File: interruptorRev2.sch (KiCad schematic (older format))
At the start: 18 parts, among them J1 220v, J2 Conn_01x04, J3 Screw_Terminal_01x03, J4 Screw_Terminal_01x03, J7 Conn_01x02, Q1 2N7002, Q2 2N7002, U1 HLK-PM01, U3 ESP-07v2, U4 JRC-21(4100), U5 JRC-21(4100)

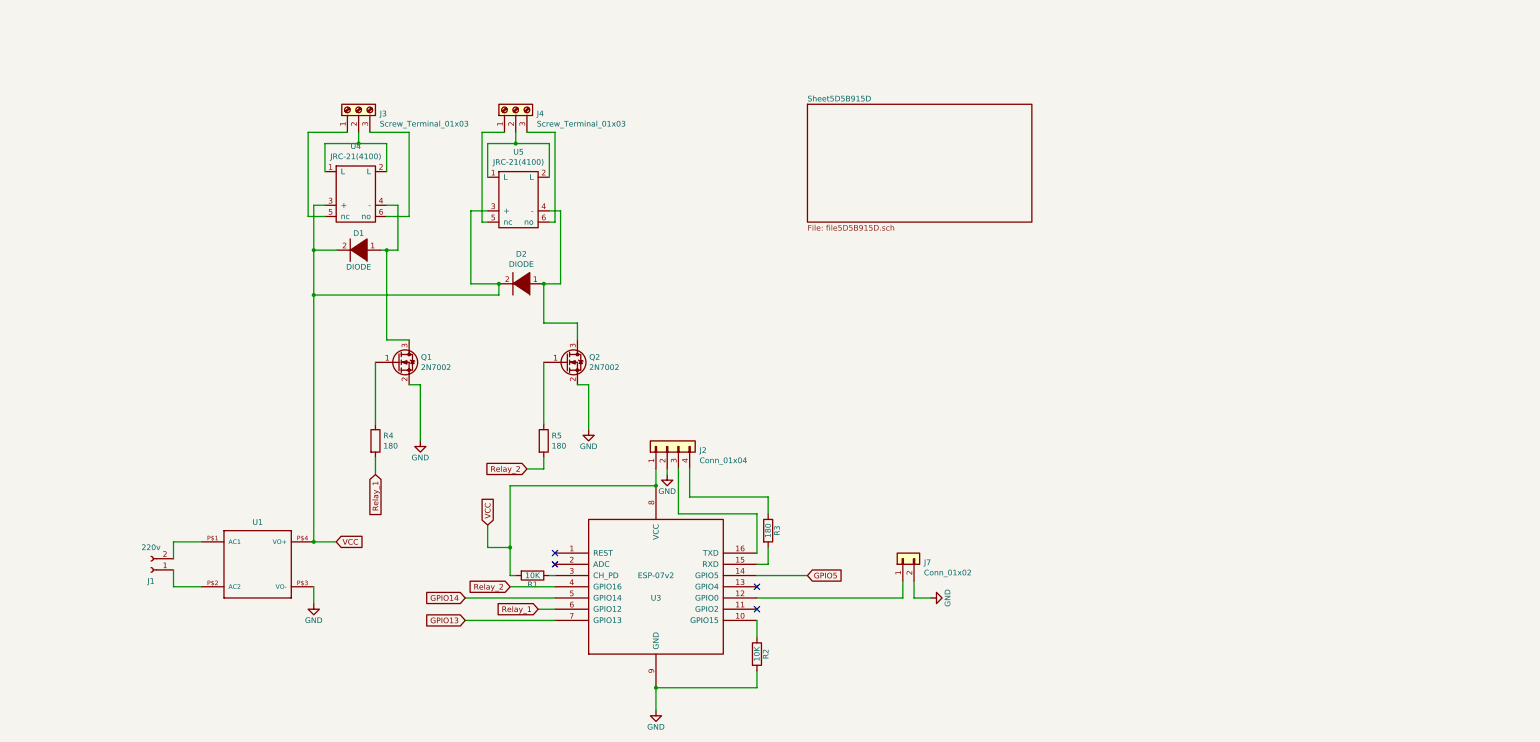
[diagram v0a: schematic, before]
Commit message: esquema dividido por secciones
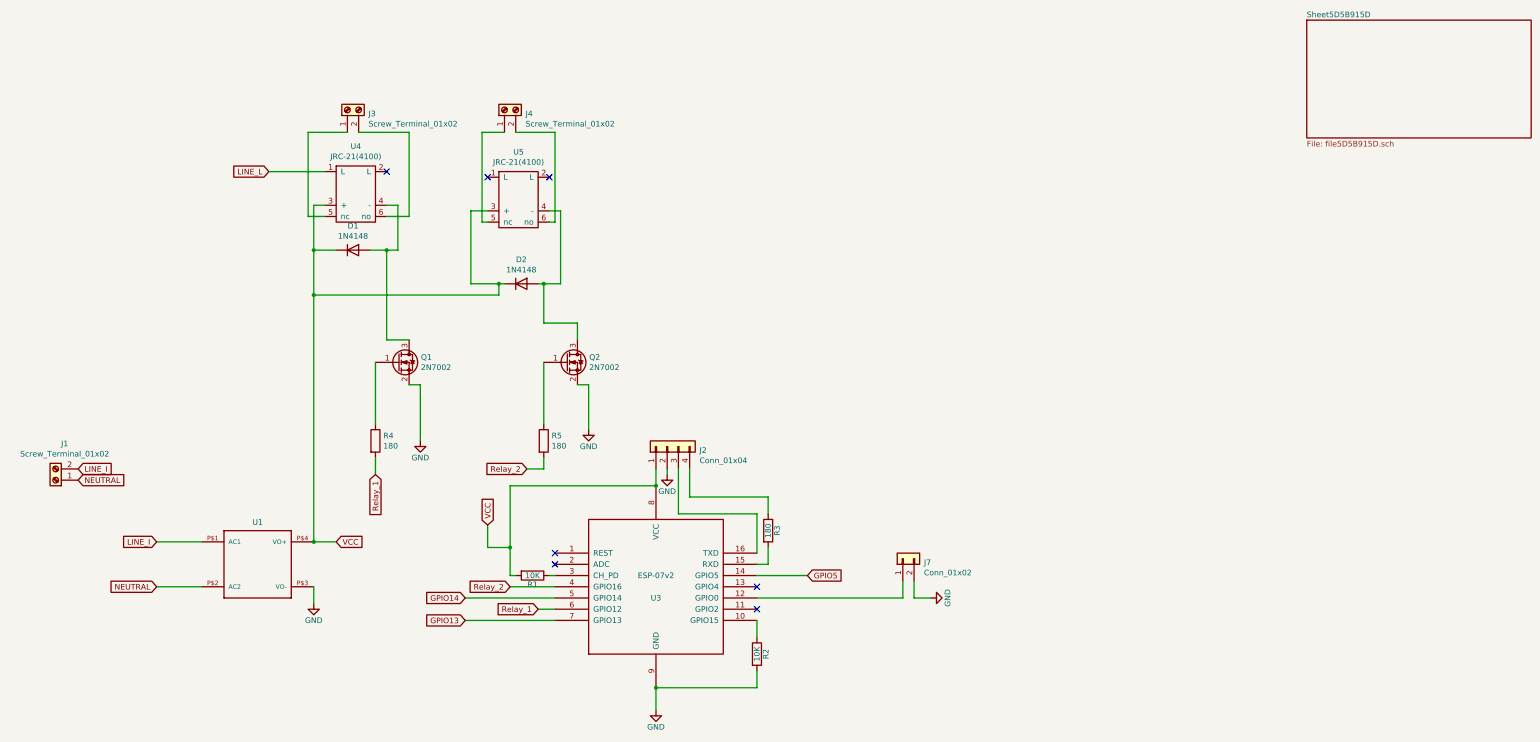
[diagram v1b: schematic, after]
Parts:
- removed D1, D2: DIODE, Diode_SMD:D_1206_3216Metric_Pad1.42x1.75mm_HandSolder, symbol pspice:DIODE
- removed J1: 220v, TerminalBlock:TerminalBlock_bornier-2_P5.08mm, symbol interruptorRev2-rescue:Conn_01x02_Female-RESCUE-termostato-termostato-rescue-in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
- removed J3, J4: Screw_Terminal_01x03, TerminalBlock:TerminalBlock_bornier-3_P5.08mm, symbol Connector:Screw_Terminal_01x03
- added D1, D2: 1N4148, espurna-h:SOD80, symbol Diode:1N4148
- added J1, J3, J4: Screw_Terminal_01x02, symbol Connector:Screw_Terminal_01x02
- R1, R2, R3, R4, R5: footprint Resistor_SMD:R_1206_3216Metric_Pad1.42x1.75mm_HandSolder -> Resistor_SMD:R_0805_2012Metric_Pad1.15x1.40mm_HandSolder
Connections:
- net VCC: now also D1.1 (K), D2.1 (K)
- net NEUTRAL: now reaches U1.P$2 (AC2)
- net NEUTRAL: now also J1.1 (Pin_1)
- net LINE_I: now reaches U1.P$1 (AC1)
- net LINE_I: now also J1.2 (Pin_2)
- net at Q1.3 (D), U4.4 (-): now also D1.2 (A)
- net at Q2.3 (D), U5.4 (-): now also D2.2 (A)
- net at U4.5 (nc): now also J3.1 (Pin_1)
- net at U4.2 (L): no longer U4.1 (L)
- net at U4.6 (no): now also J3.2 (Pin_2)
- net at U5.5 (nc): now also J4.1 (Pin_1)
- net at U5.1 (L): no longer U5.2 (L)
- net at U5.6 (no): now also J4.2 (Pin_2)
- new net LINE_L: U4.1 (L)
- no-connect marks 4 -> 7
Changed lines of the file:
@@
 Comment4 ""
 $EndDescr
-$Comp
-L interruptorRev2-rescue:Conn_01x02_Female-RESCUE-termostato-termostato-rescue-interruptor-rescue J1
-U 1 1 5A3E8B13
-P 2300 5000
-F 0 "J1" H 2300 5100 50  0000 C CNN
-F 1 "220v" H 2300 4800 50  0000 C CNN
-F 2 "TerminalBlock:TerminalBlock_bornier-2_P5.08mm" H 2300 5000 50  0001 C CNN
-F 3 "" H 2300 5000 50  0001 C CNN
-	1    2300 5000
-	-1   0    0    1
-$EndComp
 NoConn ~ 5900 4850
 NoConn ~ 5900 4950
@@
 F 0 "R3" V 7880 4650 50  0000 C CNN
 F 1 "180" V 7800 4650 50  0000 C CNN
-F 2 "Resistor_SMD:R_1206_3216Metric_Pad1.42x1.75mm_HandSolder" V 7730 4650 50  0001 C CNN
+F 2 "Resistor_SMD:R_0805_2012Metric_Pad1.15x1.40mm_HandSolder" V 7730 4650 50  0001 C CNN
 F 3 "" H 7800 4650 50  0001 C CNN
 	1    7800 4650
@@
 F 0 "R2" V 7780 5750 50  0000 C CNN
 F 1 "10K" V 7700 5750 50  0000 C CNN
-F 2 "Resistor_SMD:R_1206_3216Metric_Pad1.42x1.75mm_HandSolder" V 7630 5750 50  0001 C CNN
+F 2 "Resistor_SMD:R_0805_2012Metric_Pad1.15x1.40mm_HandSolder" V 7630 5750 50  0001 C CNN
 F 3 "" H 7700 5750 50  0001 C CNN
 	1    7700 5750
@@
 F 0 "R1" V 5780 5050 50  0000 C CNN
 F 1 "10K" V 5700 5050 50  0000 C CNN
-F 2 "Resistor_SMD:R_1206_3216Metric_Pad1.42x1.75mm_HandSolder" V 5630 5050 50  0001 C CNN
+F 2 "Resistor_SMD:R_0805_2012Metric_Pad1.15x1.40mm_HandSolder" V 5630 5050 50  0001 C CNN
 F 3 "" H 5700 5050 50  0001 C CNN
 	1    5700 5050
@@
 $EndComp
 Wire Wire Line
-	2500 4900 2500 4750
-Wire Wire Line
-	2500 5000 2500 5150
-Wire Wire Line
-	2500 5150 2750 5150
+	2350 5150 2750 5150
 Wire Wire Line
 	3750 5150 3750 5300
@@
 	1    0    0    -1
 $EndComp
-$Comp
-L pspice:DIODE D1
-U 1 1 5CD2F6F3
-P 4150 2150
-F 0 "D1" H 4150 2000 50  0000 C CNN
-F 1 "DIODE" H 4150 2300 50  0000 C CNN
-F 2 "Diode_SMD:D_1206_3216Metric_Pad1.42x1.75mm_HandSolder" H 4150 2150 50  0001 C CNN
-F 3 "~" H 4150 2150 50  0001 C CNN
-	1    4150 2150
-	-1   0    0    1
-$EndComp
-$Comp
-L pspice:DIODE D2
-U 1 1 5CD326D9
-P 5600 2450
-F 0 "D2" H 5600 2185 50  0000 C CNN
-F 1 "DIODE" H 5600 2276 50  0000 C CNN
-F 2 "Diode_SMD:D_1206_3216Metric_Pad1.42x1.75mm_HandSolder" H 5600 2450 50  0001 C CNN
-F 3 "~" H 5600 2450 50  0001 C CNN
-	1    5600 2450
-	-1   0    0    1
-$EndComp
 Wire Wire Line
 	3750 2550 5400 2550
@@
 	5400 2550 5400 2450
 Connection ~ 3750 2550
-Wire Wire Line
-	4350 2150 4400 2150
 $Comp
 L Device:R R4
@@
 F 0 "R4" H 4370 3896 50  0000 L CNN
 F 1 "180" H 4370 3805 50  0000 L CNN
-F 2 "Resistor_SMD:R_1206_3216Metric_Pad1.42x1.75mm_HandSolder" V 4230 3850 50  0001 C CNN
+F 2 "Resistor_SMD:R_0805_2012Metric_Pad1.15x1.40mm_HandSolder" V 4230 3850 50  0001 C CNN
 F 3 "~" H 4300 3850 50  0001 C CNN
 	1    4300 3850
@@
 F 0 "R5" H 5870 3896 50  0000 L CNN
 F 1 "180" H 5870 3805 50  0000 L CNN
-F 2 "Resistor_SMD:R_1206_3216Metric_Pad1.42x1.75mm_HandSolder" V 5730 3850 50  0001 C CNN
+F 2 "Resistor_SMD:R_0805_2012Metric_Pad1.15x1.40mm_HandSolder" V 5730 3850 50  0001 C CNN
 F 3 "~" H 5800 3850 50  0001 C CNN
 	1    5800 3850
@@
 Wire Wire Line
 	3750 4750 3950 4750
-$Comp
-L Connector:Screw_Terminal_01x03 J3
-U 1 1 5CD5F5C6
-P 4150 900
-F 0 "J3" V 4116 712 50  0000 R CNN
-F 1 "Screw_Terminal_01x03" V 4025 712 50  0000 R CNN
-F 2 "TerminalBlock:TerminalBlock_bornier-3_P5.08mm" H 4150 900 50  0001 C CNN
-F 3 "~" H 4150 900 50  0001 C CNN
-	1    4150 900
-	0    -1   -1   0
-$EndComp
-$Comp
-L Connector:Screw_Terminal_01x03 J4
-U 1 1 5CD62DF4
-P 5550 900
-F 0 "J4" V 5516 712 50  0000 R CNN
-F 1 "Screw_Terminal_01x03" V 5425 712 50  0000 R CNN
-F 2 "TerminalBlock:TerminalBlock_bornier-3_P5.08mm" H 5550 900 50  0001 C CNN
-F 3 "~" H 5550 900 50  0001 C CNN
-	1    5550 900
-	0    -1   -1   0
-$EndComp
 Wire Wire Line
 	7000 4100 7000 4500
@@
 	7700 5250 9000 5250
 Wire Wire Line
-	2500 4750 2750 4750
+	2350 4750 2750 4750
 $Comp
 L interruptorRev2-rescue:JRC-21(4100)-reles U4
@@
 Wire Wire Line
 	4500 1750 4500 2150
-Connection ~ 4400 2150
 Wire Wire Line
 	4600 1100 4600 1850
@@
 	4600 1850 4400 1850
 Wire Wire Line
-	4250 1100 4600 1100
+	4150 1100 4600 1100
 Wire Wire Line
 	3700 1100 3700 1850
@@
 Wire Wire Line
 	3700 1100 4050 1100
-Wire Wire Line
-	4150 1100 4150 1200
-Wire Wire Line
-	4150 1200 4400 1200
-Wire Wire Line
-	4400 1200 4400 1450
-Wire Wire Line
-	4150 1200 3850 1200
-Wire Wire Line
-	3850 1200 3850 1450
-Connection ~ 4150 1200
 $Comp
 L interruptorRev2-rescue:JRC-21(4100)-reles U5
@@
 Wire Wire Line
 	5150 2450 5400 2450
-Connection ~ 5400 2450
 Wire Wire Line
 	5850 1800 5950 1800
@@
 Wire Wire Line
 	5950 2450 5800 2450
-Connection ~ 5800 2450
 Wire Wire Line
 	5450 1100 5250 1100
@@
 	5250 1900 5300 1900
 Wire Wire Line
-	5650 1100 5900 1100
+	5550 1100 5900 1100
 Wire Wire Line
 	5900 1100 5900 1900
 Wire Wire Line
 	5900 1900 5850 1900
-Wire Wire Line
-	5300 1500 5300 1200
-Wire Wire Line
-	5300 1200 5550 1200
-Wire Wire Line
-	5550 1200 5550 1100
-Wire Wire Line
-	5850 1500 5850 1200
-Wire Wire Line
-	5850 1200 5550 1200
-Connection ~ 5550 1200
 Wire Wire Line
 	3750 2550 3750 4750
@@
 $EndComp
 $Sheet
-S 8150 850  2000 1050
+S 12600 100  2000 1050
 U 5D5B915E
 F0 "Sheet5D5B915D" 50
@@
 Text GLabel 5300 4600 1    50   Input ~ 0
 VCC
+$Comp
+L Diode:1N4148 D1
+U 1 1 5D5C40DC
+P 4100 2150
+F 0 "D1" H 4100 2366 50  0000 C CNN
+F 1 "1N4148" H 4100 2275 50  0000 C CNN
+F 2 "espurna-h:SOD80" H 4100 1975 50  0001 C CNN
+F 3 "http://www.nxp.com/documents/data_sheet/1N4148_1N4448.pdf" H 4100 2150 50  0001 C CNN
+	1    4100 2150
+	1    0    0    -1
+$EndComp
+Wire Wire Line
+	4250 2150 4400 2150
+Connection ~ 4400 2150
+$Comp
+L Diode:1N4148 D2
+U 1 1 5D5C9A7E
+P 5600 2450
+F 0 "D2" H 5600 2666 50  0000 C CNN
+F 1 "1N4148" H 5600 2575 50  0000 C CNN
+F 2 "espurna-h:SOD80" H 5600 2275 50  0001 C CNN
+F 3 "http://www.nxp.com/documents/data_sheet/1N4148_1N4448.pdf" H 5600 2450 50  0001 C CNN
+	1    5600 2450
+	1    0    0    -1
+$EndComp
+Wire Wire Line
+	5400 2450 5450 2450
+Connection ~ 5400 2450
+Wire Wire Line
+	5750 2450 5800 2450
+Connection ~ 5800 2450
+Text GLabel 1650 4200 2    50   Input ~ 0
+NEUTRAL
+Text GLabel 2350 5150 0    50   Input ~ 0
+NEUTRAL
+Text GLabel 1650 4100 2    50   Input ~ 0
+LINE_I
+Text GLabel 2350 4750 0    50   Input ~ 0
+LINE_I
+$Comp
+L Connector:Screw_Terminal_01x02 J1
+U 1 1 5D5EA3D7
+P 1450 4200
+F 0 "J1" H 1370 3875 50  0000 C CNN
+F 1 "Screw_Terminal_01x02" H 1370 3966 50  0000 C CNN
+F 2 "" H 1450 4200 50  0001 C CNN
+F 3 "~" H 1450 4200 50  0001 C CNN
+	1    1450 4200
+	-1   0    0    1
+$EndComp
+$Comp
+L Connector:Screw_Terminal_01x02 J3
+U 1 1 5D5EA93C
+P 4050 900
+F 0 "J3" V 4016 712 50  0000 R CNN
+F 1 "Screw_Terminal_01x02" V 3925 712 50  0000 R CNN
+F 2 "" H 4050 900 50  0001 C CNN
+F 3 "~" H 4050 900 50  0001 C CNN
+	1    4050 900
+	0    -1   -1   0
+$EndComp
+$Comp
+L Connector:Screw_Terminal_01x02 J4
+U 1 1 5D5ECB90
+P 5450 900
+F 0 "J4" V 5416 712 50  0000 R CNN
+F 1 "Screw_Terminal_01x02" V 5325 712 50  0000 R CNN
+F 2 "" H 5450 900 50  0001 C CNN
+F 3 "~" H 5450 900 50  0001 C CNN
+	1    5450 900
+	0    -1   -1   0
+$EndComp
+Wire Wire Line
+	3850 1450 3350 1450
+Text GLabel 3350 1450 0    50   Input ~ 0
+LINE_L
+NoConn ~ 4400 1450
+NoConn ~ 5300 1500
+NoConn ~ 5850 1500
 $EndSCHEMATC
